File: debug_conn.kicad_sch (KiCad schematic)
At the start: 16 parts, among them CN1 HX JN1.27-2X5P ZZ H4.9, J3 Conn_01x06_Pin, U14 TXU0202DCUR

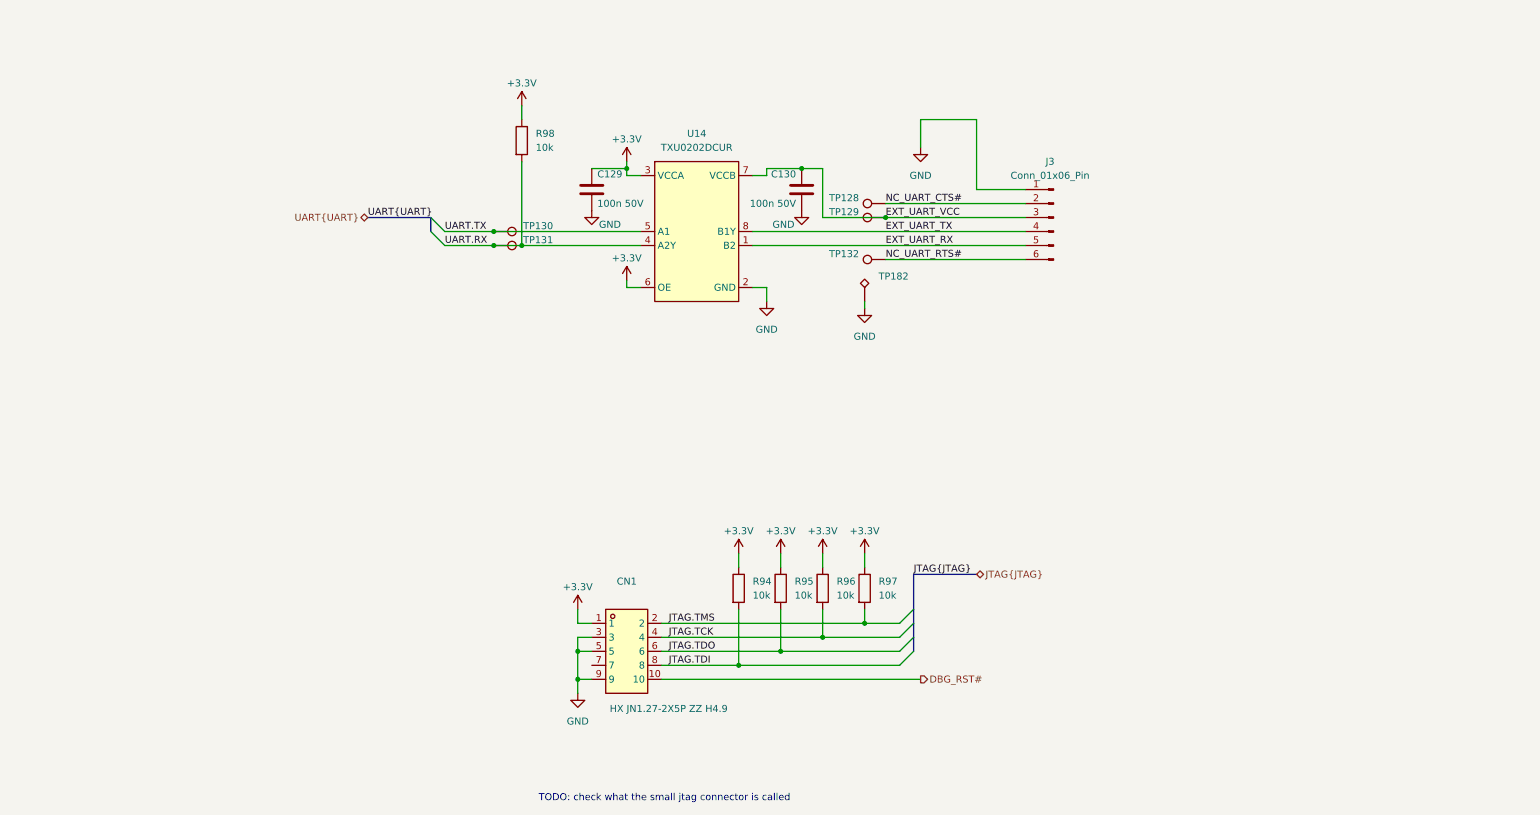
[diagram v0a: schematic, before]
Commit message: did stuff
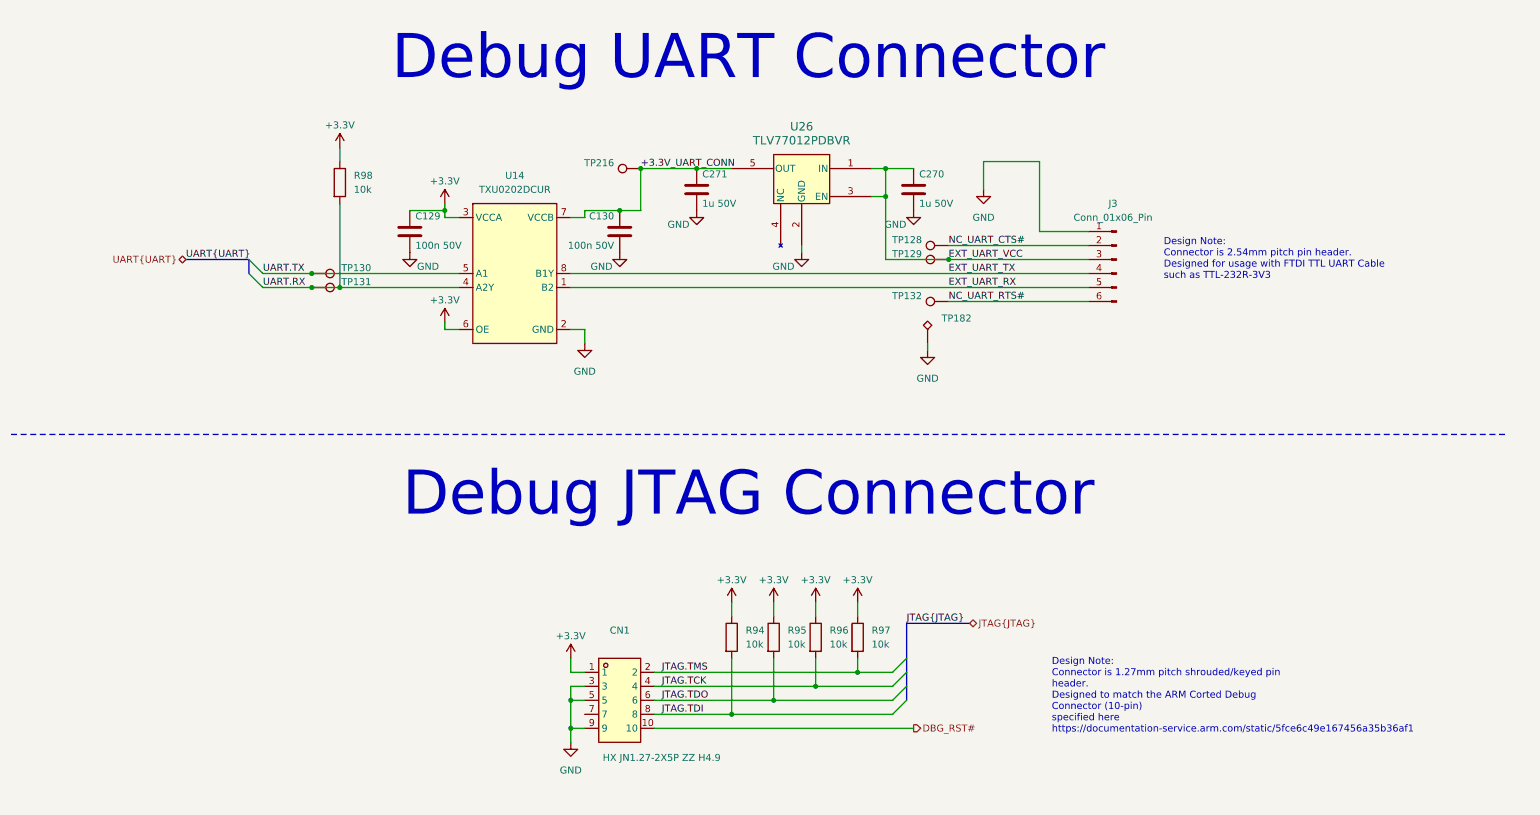
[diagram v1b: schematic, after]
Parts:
- added C270, C271: 1u 50V, Capacitor_SMD:C_0603_1608Metric, symbol Device:C
- added TP216: TestPoint, TestPoint:TestPoint_THTPad_D1.0mm_Drill0.5mm, symbol Connector:TestPoint
- added U26: TLV77012PDBVR, TLV770:SOT-23-5_DBV_TEX, symbol TLV770:TLV77012PDBVR
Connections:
- net EXT_UART_VCC: now also C270.1, U26.1 (IN), U26.3 (EN); no longer C130.1, U14.7 (VCCB)
- net GND: now also C270.2, C271.2, U26.2 (GND)
- new net +3.3V_UART_CONN: C130.1, C271.1, TP216.1, U14.7 (VCCB), U26.5 (OUT)
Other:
- note added: "Debug JTAG Connector"
- note added: "Debug UART Connector"
- note removed: "TODO: check what the small jtag connector is called"
- moved on the sheet: C129, C130, CN1, J3, R94, R95, R96, R97, R98, TP128, TP129, TP130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
